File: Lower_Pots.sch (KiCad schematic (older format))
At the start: 17 parts, among them U5 CD74HC4067M

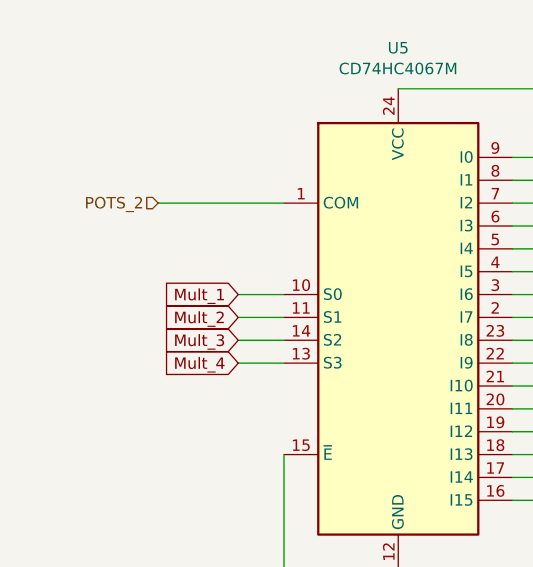
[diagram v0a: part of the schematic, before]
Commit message: Sub boards completed
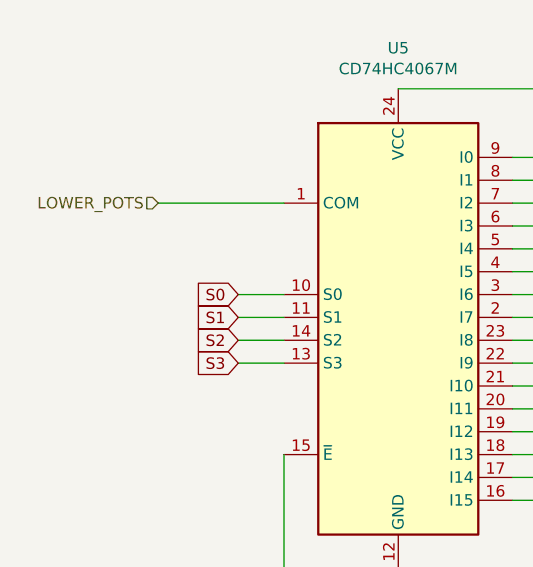
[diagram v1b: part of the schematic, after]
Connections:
- net Mult_1 renamed S0
- net Mult_2 renamed S1
- net Mult_3 renamed S2
- net Mult_4 renamed S3
- net POTS_2 renamed LOWER_POTS
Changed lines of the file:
@@
 Connection ~ 2700 7100
 Text HLabel 1650 1900 0    50   Input ~ 0
-POTS_2
+LOWER_POTS
 Wire Wire Line
 	1650 1900 2200 1900
-Text GLabel 2000 2600 0    50   Input ~ 0
-Mult_4
 Wire Wire Line
 	2000 2600 2200 2600
-Text GLabel 2000 2300 0    50   Input ~ 0
-Mult_1
-Text GLabel 2000 2400 0    50   Input ~ 0
-Mult_2
-Text GLabel 2000 2500 0    50   Input ~ 0
-Mult_3
 Wire Wire Line
 	2000 2300 2200 2300
@@
 Wire Wire Line
 	4800 1150 4800 1400
+Text GLabel 2000 2300 0    50   Input ~ 0
+S0
+Text GLabel 2000 2400 0    50   Input ~ 0
+S1
+Text GLabel 2000 2500 0    50   Input ~ 0
+S2
+Text GLabel 2000 2600 0    50   Input ~ 0
+S3
 $EndSCHEMATC
